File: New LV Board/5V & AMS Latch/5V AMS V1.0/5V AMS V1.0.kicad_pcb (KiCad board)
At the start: 2 copper layers, 46 x 64.5 mm, 19 parts, among them J2 B12B-PH-K-S, J4 691137710002, J6 PH1-20-UA, J9 PH1-20-UA, K1 AHES4291, SW1 Test Reset AMS, U1 LT1117-5.0

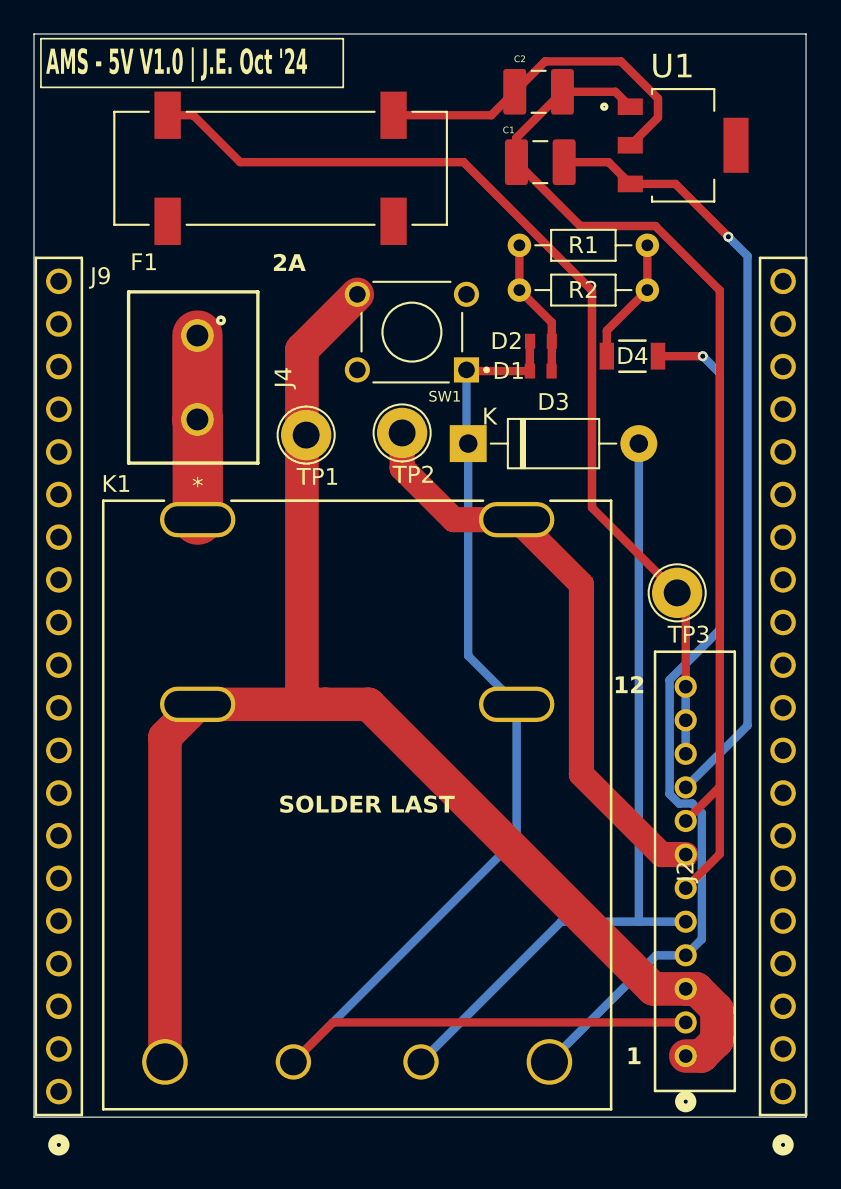
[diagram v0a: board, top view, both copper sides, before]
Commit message: PCB cleanup and retrace
PCB cleanup and retrace
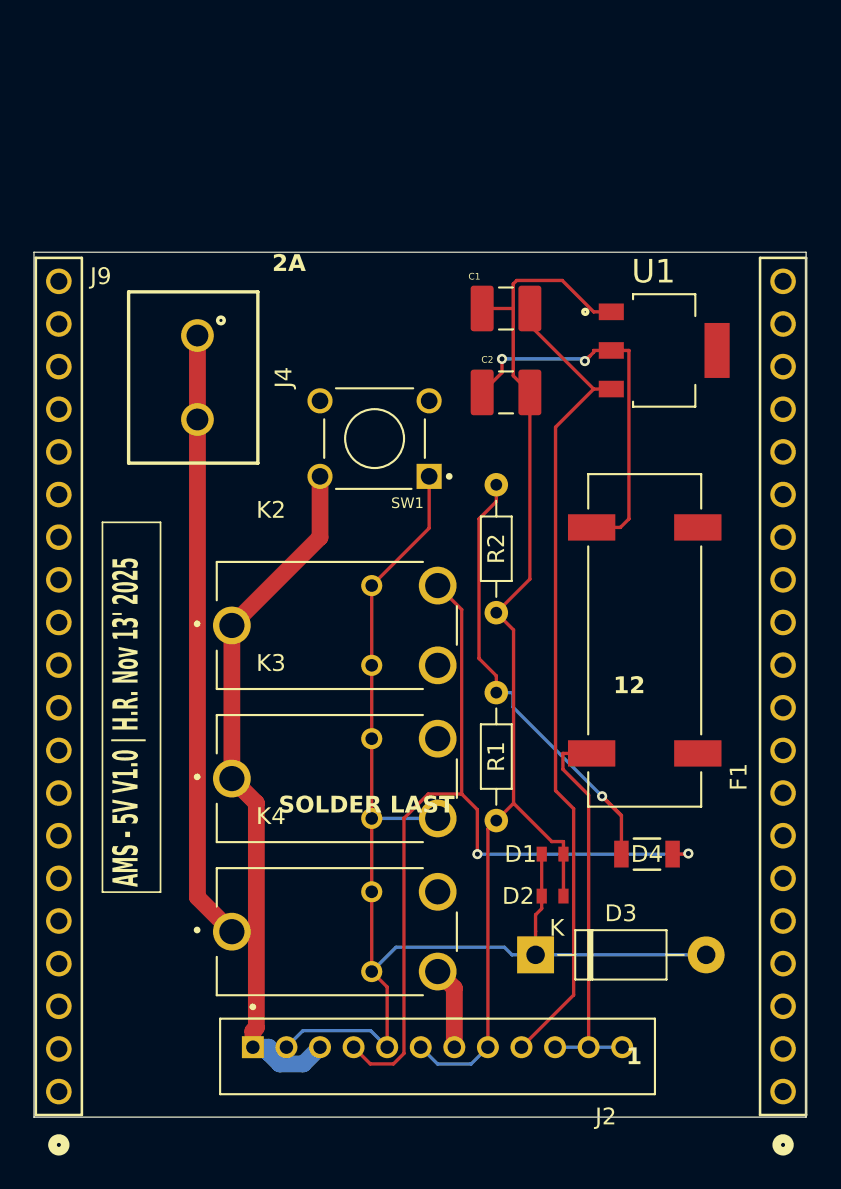
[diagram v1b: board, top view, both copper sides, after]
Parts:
- removed K1: AHES4291, motorSports:AHES4_PAN
- removed TP1, TP2, TP3: TestPoint, TestPoint:TestPoint_Loop_D2.60mm_Drill1.6mm_Beaded
- added K2: A161CS12VDC.64, Footprints:RELAY_A161CS12VDC.64, F.Cu at (76.5, 140.9)
- added K3: A161CS12VDC.64, Footprints:RELAY_A161CS12VDC.64, F.Cu at (76.5, 150.0)
- added K4: A161CS12VDC.64, Footprints:RELAY_A161CS12VDC.64, F.Cu at (76.5, 159.1)
- J2: footprint MotorSports_KICad:CONN12_B12B-PH_JST -> Footprints:JST_B12B-PH-K-S
- moved F1 35.5 mm to (94.8, 141.8), turned to 90 degrees
- moved R1 34.3 mm to (86.0, 152.5), turned to 90 degrees
- moved D2 33.1 mm to (89.4, 157.0)
- moved D3 30.7 mm to (88.3, 160.5)
- moved D4 29.7 mm to (95.0, 154.5)
- moved D1 28.8 mm to (89.4, 154.5)
- moved R2 19.3 mm to (86.0, 140.1), turned to 90 degrees
- moved C2 18.0 mm to (86.6, 127.0)
- moved J2 14.8 mm to (82.5, 166.6), turned to 180 degrees
- moved U1 12.3 mm to (96.0, 124.5)
- moved C1 8.95 mm to (86.6, 122.0)
- moved SW1 6.72 mm to (78.8, 129.8)
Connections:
- D3 pad 2: Net-(D3-A) -> Net-(D1-K)
- J2 pad 5: Net-(D3-A) -> Net-(D1-K)
- SW1 pad 2: (no net) -> Net-(J2-Pad1)
- SW1 pad 4: Net-(J2-Pad1) -> (no net)
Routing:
- net Net-(J2-Pad1): track 90.4 -> 41.9 mm
- net Net-(D3-A): track 47.7 -> 0.00 mm
- net Net-(F1-Pad1_1): track 59.7 -> 23.8 mm
- net Net-(J2-Pad7): track 35.1 -> 4.92 mm
- net Net-(D4-K): track 7.60 -> 33.0 mm, vias 0 -> 1
- net Net-(J4-Pad1): track 11.0 -> 36.4 mm
- net Net-(D1-K): track 77.9 -> 73.4 mm
- net /GND: track 72.6 -> 68.3 mm
- net Net-(U1-VO): track 21.5 -> 24.6 mm, vias 0 -> 2
- net /Vs: track 46.4 -> 49.3 mm, vias 1 -> 0
- net Net-(D4-A): track 52.4 -> 52.2 mm, vias 1 -> 2
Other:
- board size 46 x 64.5 mm -> 46 x 51.5 mm
- board text added: "AMS - 5V V1.0 | H.R. Nov 13' 2025"
- board text removed: "AMS - 5V V1.0 | J.E. Oct '24"
